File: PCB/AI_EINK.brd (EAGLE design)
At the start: 66 x 111.6 mm, 186 parts, among them IC3 WM8960, J1 BM04B-GHS-TBT(LF)(SN)(N), J2 C393939, J3 524372471, Q1 SI1308EDL-T1-GE3, Q3 NMOS_C7465427, T1 MMUN2133LT1G, U1 TPS61092RSAR, U10 AP2112-3.3K, U11 AP2112-3.3K, U12 SPU0410LR5H-QB, U2 MC74VHC1G14DFT1G, U3 BQ27441DRZR-G1A, U4 BQ24075, U5 TLV74328, U6 TLV74315, U7 TLV74318PDBVRDBV0005A_L, U8 ST25DV64K-IER6S3SOIC_IER6S3_S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, U9 EMC2301-1-ACZL-TRMSOP8_MC_MCH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, Y1 ABM8-272-T3

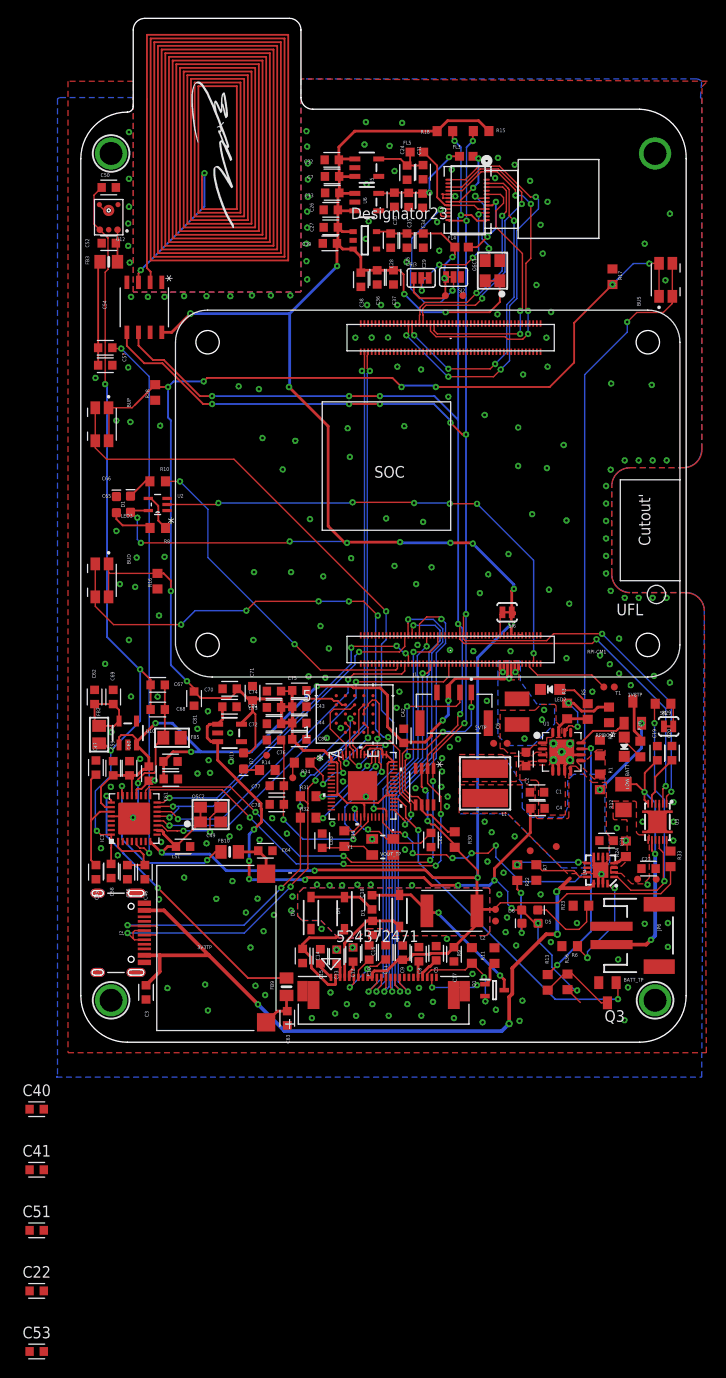
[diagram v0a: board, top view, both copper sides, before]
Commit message: PCB V3
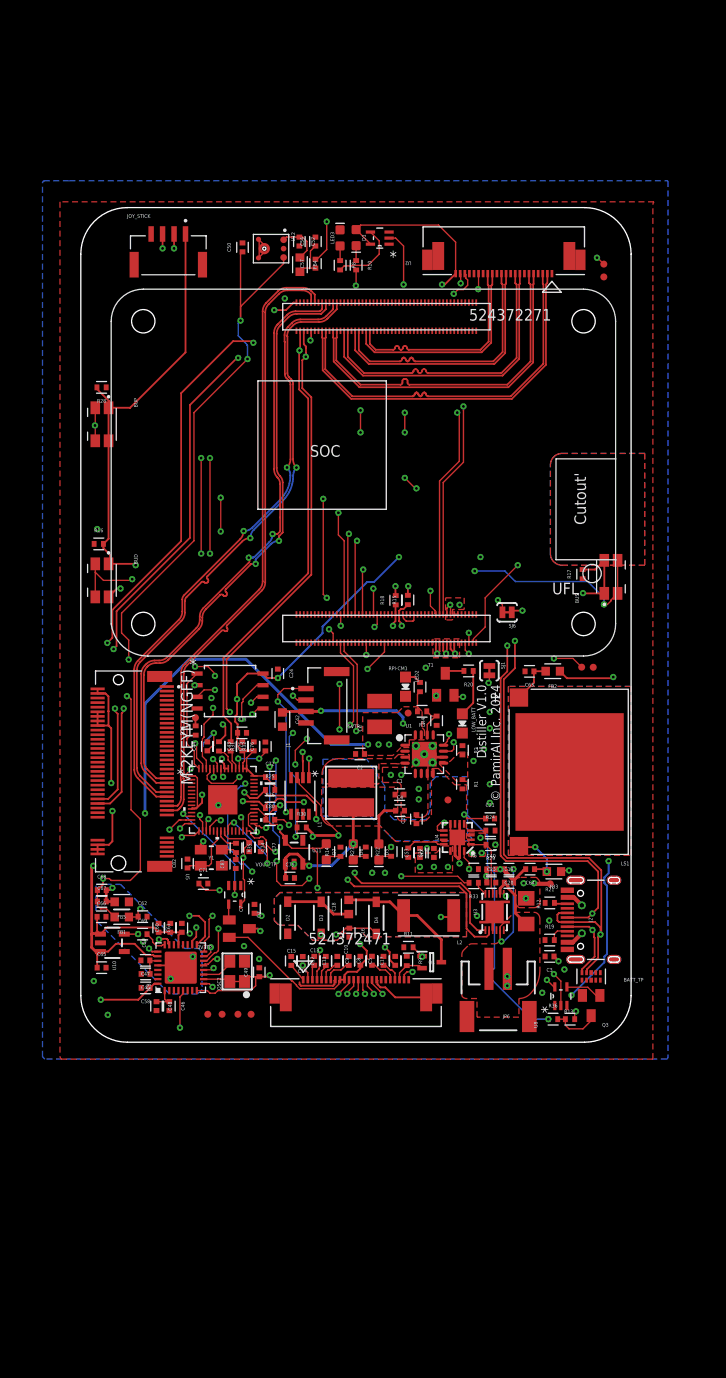
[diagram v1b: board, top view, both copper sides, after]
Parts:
- removed ANT1: NFC_ANTENNA_25X15, microbuilder:NFCANT_25X15
- removed C25, C30: 1.0uF, Capacitor:CAPC1608X85
- removed C27, C70, C78, C81: 0.1uF, Capacitor:CAPC1608X85
- removed C28, C29, C31, C32, C33, C34, C35, C36, C37, C38, C39, C41, C51: 10uF, Capacitor:CAPC1608X85
- removed FB10, FB9: 120o, microbuilder:0805-NO
- removed FL3, FL4, FL5: BLM18HE152SN1D, BLM18HE152SN1D:BEADC1608X95N
- removed GND25, RPIBOOT3: DNP, SparkFun-Connectors:PAD.03X.03
- removed J3: 524372471, 2024-02-19_09-48-43_Library:CON_524372471_MOL
- removed OSC1: 24MHz 3.3V Oscillator, microbuilder:OSC_3.2X2.5MM
- removed OV5674: DF30FC-24DS-0.4V(82)CONN_DF30FC-24DS-0.4V(82)_HIR, 2024-03-07_05-07-01_Library:CONN_DF30FC-24DS-0.4V(82)_HIR
- removed SJ2, SJ3: DNP, SparkFun-Passives:PAD-JUMPER-3-2OF3_NC_BY_TRACE_YES_SILK_FULL_BOX
- removed SPI_FLASH_SAM: W25Q128JVBIQTFBGA_128JVBIQ_WIN, 2024-03-10_02-04-46_Library:TFBGA_128JVBIQ_WIN
- removed U$10, U$11, U$94, U$95: MOUNTINGHOLE2.5, microbuilder:MOUNTINGHOLE_2.5_PLATED
- removed U7: TLV74318PDBVRDBV0005A_L, 2024-03-10_03-34-55_Library:DBV0005A_L
- added CAMERA: 524372271CON_524372271_MOL, 2024-03-29_02-21-27_Library:CON_524372271_MOL
- added EINK_524352471: 524372471, 2024-02-19_09-48-43_Library:CON_524372471_MOL
- added FB1, FB4: FERRITE_BEAD, Filter:BEADC1608X95N
- added JOY_STICK: BM04B-GHS-TBT(LF)(SN)(N), BM04B-GHS-TBT_LF__SN__N_:JST_BM04B-GHS-TBT(LF)(SN)(N)
- added M.2KEYM(NGFF): 1-2199119-5, 1-2199119-5:TE_1-2199119-5
- added Q2: NMOS_C7465427, Transistor:SOT23
- added R19: 5.1K, Resistor:RESC1005X40
- added R21: 5.1k, Resistor:RESC1005X40
- added R25, R26: 4.7K, Resistor:RESC1005X40
- added U13: TPD4EUSB30DQARDQA10, 2024-03-29_01-35-38_Library:DQA10
- C1, C10, C11, C12, C13, C14, C15, C16, C17, C19, C2, C20, C21, C22, C23, C26, C3, C4, C40, C43, C44, C45, C46, C47, C48, C49, C5, C50, C52, C53, C54, C57, C58, C59, C60, C61, C62, C63, C64, C65, C66, C67, C68, C69, C7, C71, C72, C73, C74, C75, C76, C77, C79, C8, C80, C82, C83, C9: device Capacitor:CAPC1608X85 -> Capacitor:CAPC1005X60
- C24: value 10uF -> 0.1uF; device Capacitor:CAPC1608X85 -> Capacitor:CAPC1005X60
- FB2, FB5: value Ferrite -> FERRITE_BEAD; device microbuilder:0805 -> Filter:BEADC1608X95N
- FB3: value Ferrite -> FERRITE_BEAD; device microbuilder:0805-NO -> Filter:BEADC1608X95N
- R1, R10, R11, R13, R14, R15, R16, R17, R18, R2, R20, R22, R23, R24, R28, R29, R3, R30, R31, R32, R33, R34, R35, R36, R4, R5, R6, R7, R8, R9: device resistor:R0603 -> Resistor:RESC1005X40
- U5: value TLV74328 -> MC74VHC1G14DFT1G; device adafruit_power:SOT23-5 -> MC74VHC1G14DFT1G:SOT65P210X110-5N
- U6: value TLV74315 -> W25Q128JVSIQSOIC_128JVSIQ_WIN-L; device adafruit_power:SOT23-5 -> 2024-03-29_04-43-21_Library:SOIC_128JVSIQ_WIN-L
- U8: value ST25DV64K-IER6S3SOIC_IER6S3_STM -> MC74VHC1G14DFT1G; device 2024-03-10_23-40-44_Library:SOIC_IER6S3_STM -> MC74VHC1G14DFT1G:SOT65P210X110-5N
- moved U8 87.8 mm to (53.3, 9.02), turned to 90 degrees
- moved FB3 82.3 mm to (52.6, 22.6)
- moved U5 80.6 mm to (17.8, 20.1)
- moved C7 80.3 mm to (19.9, 18.5), turned to 90 degrees
- moved RPIBOOT2 71.3 mm to (58.0, 88.8)
- moved C53 68.6 mm to (38.0, 24.6), turned to 90 degrees
- moved C26 67.1 mm to (37.6, 28.3), turned to 90 degrees
- moved GND13 65.9 mm to (58.0, 87.4)
- moved C22 64.5 mm to (39.5, 24.6), turned to 90 degrees
- moved GND 56.9 mm to (14.8, 7.05)
- moved C24 56.4 mm to (22.5, 44.2)
- moved C40 56.0 mm to (45.7, 22.9)
- moved U6 55.4 mm to (17.3, 42.3), turned to 0 degrees
- moved R15 51.7 mm to (36.7, 52.2), turned to 90 degrees
- moved R18 51.4 mm to (35.3, 52.2), turned to 90 degrees
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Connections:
- removed net 1.5V: C30.1, C34.1, C35.1, FL3.1, U6.5
- removed net 1.8V: C25.1, C28.1, C29.1, FL4.1, RPIBOOT3.P$1, SJ2.3, SJ3.1, U7.5
- removed net 2.8V: C24.1, C31.1, FL5.1, U5.5
- removed net AF_EN: OV5674.18
- removed net GPO: U8.7
- removed net N$10: FL4.2, OV5674.15
- removed net N$13: FL3.2, OV5674.13, OV5674.14
- removed net N$20: RPI-CM1.29
- removed net N$22: RPI-CM1.41
- removed net N$28: RPI-CM1.55
- removed net N$32: ANT1.P$1, U8.3
- removed net PWDN: OV5674.19, SJ3.2
- removed net RESET: OV5674.22, SJ2.2
- removed net RFC_MCLK: OSC1.3, OV5674.11
- removed net SAM_GPIO0: C2040.2
- removed net SAM_GPIO10: C2040.13
- removed net SAM_GPIO11: C2040.14
- removed net SAM_GPIO12: C2040.15
- removed net SAM_GPIO13: C2040.16
- removed net SAM_GPIO14: C2040.17
- removed net SAM_GPIO15: C2040.18
- removed net SAM_GPIO23: C2040.35
- removed net SAM_GPIO24: C2040.36
- removed net SAM_GPIO9: C2040.12
- removed net SCL: IC3.17, OV5674.23, R18.1, RPI-CM1.56, U3.2, U8.6, U9.2
- removed net SDA: IC3.18, OV5674.24, R15.1, RPI-CM1.58, U3.1, U8.5, U9.1
- removed net STROBE: OV5674.20
- removed net SYS_POW_SAM: C2040.32, Q3.1
- removed net VEH: U8.1
- new net 3V3_EINK: C17.1, C9.1, EINK_524352471.10, EINK_524352471.9, L2.1, Q2.2
- new net CAM1_C_N: CAMERA.8, RPI-CM1.127
- new net CAM1_C_P: CAMERA.9, RPI-CM1.129
- new net CAM1_D0_N: CAMERA.2, RPI-CM1.115
- new net CAM1_D0_P: CAMERA.3, RPI-CM1.117
- new net CAM1_D1_N: CAMERA.5, RPI-CM1.121
- new net CAM1_D1_P: CAMERA.6, RPI-CM1.123
- new net CAM1_D2_N: CAMERA.11, RPI-CM1.133
- new net CAM1_D2_P: CAMERA.12, RPI-CM1.135
- new net CAM1_D3_N: CAMERA.14, RPI-CM1.139
- new net CAM1_D3_P: CAMERA.15, RPI-CM1.141
- new net DSI0_C_N: RPI-CM1.169
- new net DSI0_C_P: RPI-CM1.171
- new net DSI0_D0_N: RPI-CM1.157
- new net DSI0_D0_P: RPI-CM1.159
- new net DSI0_D1_N: RPI-CM1.163
- new net DSI0_D1_P: RPI-CM1.165
- new net DSI1_C_N: RPI-CM1.187
- new net DSI1_C_P: RPI-CM1.189
- new net DSI1_D0_N: RPI-CM1.175
- new net DSI1_D0_P: RPI-CM1.177
- new net DSI1_D1_N: RPI-CM1.181
- new net DSI1_D1_P: RPI-CM1.183
- new net DSI1_D2_N: RPI-CM1.193
- new net DSI1_D2_P: RPI-CM1.195
- new net DSI1_D3_N: RPI-CM1.194
- new net DSI1_D3_P: RPI-CM1.196
- new net EXT_VCC_PCIE: M.2KEYM(NGFF).12, M.2KEYM(NGFF).14, M.2KEYM(NGFF).16, M.2KEYM(NGFF).18, M.2KEYM(NGFF).2, M.2KEYM(NGFF).4, M.2KEYM(NGFF).70, M.2KEYM(NGFF).72, M.2KEYM(NGFF).74
- new net GND_2: U13.3
- new net HDMI0_CEC: RPI-CM1.151
- new net HDMI0_CLK_N: RPI-CM1.190
- new net HDMI0_CLK_P: RPI-CM1.188
- new net HDMI0_HOTPLUG: RPI-CM1.153
- new net HDMI0_SCL: RPI-CM1.200
- new net HDMI0_SDA: RPI-CM1.199
- new net HDMI0_TX0_N: RPI-CM1.184
- new net HDMI0_TX0_P: RPI-CM1.182
- new net HDMI0_TX1_N: RPI-CM1.178
- new net HDMI0_TX1_P: RPI-CM1.176
- new net HDMI0_TX2_N: RPI-CM1.172
- new net HDMI0_TX2_P: RPI-CM1.170
- new net HDMI1_CEC: RPI-CM1.149
- new net HDMI1_CLK_N: RPI-CM1.166
- new net HDMI1_CLK_P: RPI-CM1.164
- new net HDMI1_HOTPLUG: RPI-CM1.143
- new net HDMI1_SCL: RPI-CM1.147
- new net HDMI1_SDA: RPI-CM1.145
- new net HDMI1_TX0_N: RPI-CM1.160
- new net HDMI1_TX0_P: RPI-CM1.158
- new net HDMI1_TX1_N: RPI-CM1.154
- new net HDMI1_TX1_P: RPI-CM1.152
- new net HDMI1_TX2_N: RPI-CM1.148
- new net HDMI1_TX2_P: RPI-CM1.146
- new net N$27: J2.B5, R21.2
- new net N$30: J2.A5, R19.2
- new net PCIE_!RST: M.2KEYM(NGFF).50, RPI-CM1.109
- new net PCIE_CLK_!REQ: M.2KEYM(NGFF).52, RPI-CM1.102
- new net PCIE_CLK_N: M.2KEYM(NGFF).53, RPI-CM1.112
- new net PCIE_CLK_P: M.2KEYM(NGFF).55, RPI-CM1.110
- new net PCIE_RX_N: M.2KEYM(NGFF).41, RPI-CM1.118
- new net PCIE_RX_P: M.2KEYM(NGFF).43, RPI-CM1.116
- new net PCIE_TX_N: M.2KEYM(NGFF).47, RPI-CM1.124
- new net PCIE_TX_P: M.2KEYM(NGFF).49, RPI-CM1.122
- new net RESERVED@104: RPI-CM1.104
- new net RESERVED@106: RPI-CM1.106
- new net SAM_EINK_ON: C2040.12, U5.2
- new net SAM_INTERUPT: C2040.2, RPI-CM1.46
- new net SAM_SCL: C2040.35, JOY_STICK.3, R26.1, U3.2
- new net SAM_SDA: C2040.36, JOY_STICK.2, R25.1, U3.1
- new net SCL0: CAMERA.20, RPI-CM1.80
- new net SCL1: IC3.17, R18.1, RPI-CM1.56, U9.2
- new net SDA0: CAMERA.21, RPI-CM1.82
- new net SDA1: IC3.18, R15.1, RPI-CM1.58, U9.1
- new net SYS_PI_ON: C2040.32, U8.2
- new net USB_OTG_ID: RPI-CM1.101
- new net VDAC_COMP: RPI-CM1.111
- net 3.3V: now also CAMERA.22, Q2.3; no longer C17.1, C26.1, C27.1, C32.1, C33.1, C36.1, C37.1, C38.1, C39.1, C9.1, J3.10, J3.9, L2.1, OSC1.1, OSC1.4, U5.1, U5.3, U6.1, U6.3, U7.1, U7.3, U8.8
- net AGND: now also FB5.2; no longer FB5.1
- net AVDD: now also FB1.2; no longer FB2.1
- net CAM0_C_N: no longer OV5674.8
- net CAM0_C_P: no longer OV5674.9
- net CAM0_D0_N: no longer OV5674.2
- net CAM0_D0_P: no longer OV5674.3
- net CAM0_D1_N: no longer OV5674.5
- net CAM0_D1_P: no longer OV5674.6
- net CAM_GPIO: now also CAMERA.17
- net CDD: now also EINK_524352471.7; no longer J3.7
- net EINK_BUSY: now also C2040.13, EINK_524352471.16; no longer J3.16
- net EINK_CS: now also C2040.16, EINK_524352471.13; no longer J3.13
- net EINK_D/C: now also C2040.15, EINK_524352471.14; no longer J3.14
- net EINK_RESET: now also C2040.14, EINK_524352471.15; no longer J3.15
- net GDR: now also EINK_524352471.23; no longer J3.23
- net GND: now also C24.1, CAMERA.1, CAMERA.10, CAMERA.13, CAMERA.16, CAMERA.19, CAMERA.4, CAMERA.7, EINK_524352471.17, EINK_524352471.8, EINK_524352471.P1, EINK_524352471.P2, FB5.1, JOY_STICK.4, M.2KEYM(NGFF).1, M.2KEYM(NGFF).15, M.2KEYM(NGFF).21, M.2KEYM(NGFF).27, M.2KEYM(NGFF).3, M.2KEYM(NGFF).33, M.2KEYM(NGFF).39, M.2KEYM(NGFF).45, M.2KEYM(NGFF).51, M.2KEYM(NGFF).57, M.2KEYM(NGFF).71, M.2KEYM(NGFF).73, M.2KEYM(NGFF).75, M.2KEYM(NGFF).9, M.2KEYM(NGFF).SH1, M.2KEYM(NGFF).SH2, R19.1, R21.1, U13.8, U5.3, U6.4, U8.3; no longer C24.2, C25.2, C27.2, C28.2, C29.2, C30.2, C31.2, C32.2, C33.2, C34.2, C35.2, C36.2, C37.2, C38.2, C39.2, C41.2, C51.2, C70.2, C78.2, C81.2, FB5.2, GND25.P$1, J3.17, J3.8, J3.P1, J3.P2, OSC1.2, OV5674.1, OV5674.10, OV5674.12, OV5674.21, OV5674.4, OV5674.7, SJ2.1, SJ3.3, SPI_FLASH_SAM.B3, U5.2, U6.2, U7.2, U8.4
- net LEFT_N: now also FB3.2; no longer FB10.2
- net LEFT_P: now also FB2.2; no longer FB9.2
- net N$16: now also Q3.1, U8.4; no longer ANT1.P$2, U8.2
- net N$29: now also FB4.1; no longer FB3.1
- net N$36: now also FB4.2; no longer FB3.2
- net N$40: now also FB2.1; no longer FB9.1
- net N$41: now also FB3.1; no longer FB10.1
- net N$8: now also Q2.1, U5.4; no longer FL5.2, OV5674.16, OV5674.17
- net NC: now also EINK_524352471.24; no longer J3.24
- net OUT: now also FB1.1; no longer FB2.2
- net PREVGH: now also EINK_524352471.4; no longer J3.4
- net PREVGL: now also EINK_524352471.2; no longer J3.2
- net RESE: now also EINK_524352471.22; no longer J3.22
- net SAM_1V1: no longer C78.1
- net SAM_3V3: now also C24.2, JOY_STICK.1, R25.2, R26.2, U5.5, U6.8, U8.5; no longer C70.1, C81.1, SPI_FLASH_SAM.B4
- net SAM_QSPI_SCLK: now also U6.6; no longer SPI_FLASH_SAM.B2
- net SAM_QSPI_SCN: now also U6.1; no longer SPI_FLASH_SAM.C2
- net SAM_QSPI_SD0: now also U6.5; no longer SPI_FLASH_SAM.D3
- net SAM_QSPI_SD1: now also U6.2; no longer SPI_FLASH_SAM.D2
- net SAM_QSPI_SD2: now also U6.3; no longer SPI_FLASH_SAM.C4
- net SAM_QSPI_SD3: now also U6.7; no longer SPI_FLASH_SAM.D4
- net SPI_CLK: now also C2040.17, EINK_524352471.12; no longer J3.12
- net SPI_MOSI: now also C2040.18, EINK_524352471.11; no longer J3.11
- net TSCL: now also EINK_524352471.19; no longer J3.19
- net TSDA: now also EINK_524352471.18; no longer J3.18
- net USB_N: now also U13.5
- net USB_P: now also U13.4
- net VCOM: now also EINK_524352471.1; no longer J3.1
- net VGH: now also EINK_524352471.20; no longer J3.20
- net VGL: now also EINK_524352471.21; no longer J3.21
- net VOUT: now also C26.1
- net VPP: now also EINK_524352471.6; no longer J3.6
- net VSH: now also EINK_524352471.5; no longer J3.5
- net VSL: now also EINK_524352471.3; no longer J3.3
- net V_BATT: no longer C41.1, C51.1
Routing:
- net 3.3V: track 308.1 -> 65.7 mm, vias 19 -> 15
- net SDA: track 201.4 -> 0.00 mm, vias 15 -> 0
- net SCL: track 199.3 -> 0.00 mm, vias 13 -> 0
- net RINPUT1: track 59.4 -> 185.6 mm
- net SAM_SCL: track 0.00 -> 106.1 mm, vias 0 -> 6
- net SAM_SDA: track 0.00 -> 104.0 mm, vias 0 -> 6
- net EINK_CS: track 39.7 -> 130.5 mm, vias 2 -> 3
- net EINK_BUSY: track 49.3 -> 133.9 mm, vias 2 -> 3
- net EINK_RESET: track 49.6 -> 128.3 mm, vias 2 -> 3
- net EINK_D/C: track 47.4 -> 125.7 mm, vias 2 -> 3
- net SPI_CLK: track 42.9 -> 119.8 mm, vias 2 -> 3
- net SPI_MOSI: track 44.9 -> 118.7 mm, vias 2 -> 3
- net VBUS: track 80.3 -> 9.33 mm, vias 4 -> 6
- net PCIE_!RST: track 0.00 -> 69.0 mm, vias 0 -> 4
- net PCIE_CLK_!REQ: track 0.00 -> 67.8 mm, vias 0 -> 4
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- added copper zone on layer 1, net 3.3V
- added copper zone on layer 15, net 3.3V
- added copper zone on layer 15, net 5.0V
- added copper zone on layer 16, net AGND
- added copper zone on layer 1, net BATTERY_IN
- added copper zone on layer 2, net GND
- added copper zone on layer 15, net GND1
- added copper zone on layer 2, net GND2
- added copper zone on layer 1, net GND3
- added copper zone on layer 2, net GND4
- added copper zone on layer 15, net GND5
- added copper zone on layer 16, net GND6
- added copper zone on layer 15, net SAM_3V3
- added copper zone on layer 1, net VBUS
- added copper zone on layer 15, net VBUS
- added copper zone on layer 15, net V_BATT
- removed copper zone on layer 16, net 5.0V
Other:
- board size 66 x 111.6 mm -> 60 x 91 mm
- board text added: "Distiller V1.0 © PamirAI Inc. 2024"
- board text removed: "1V8TP"
- board text removed: "RPIBOOT"
- board text removed: "Reveri H1 V1.0 © PamirAI Inc. 2024"

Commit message: pcb v4
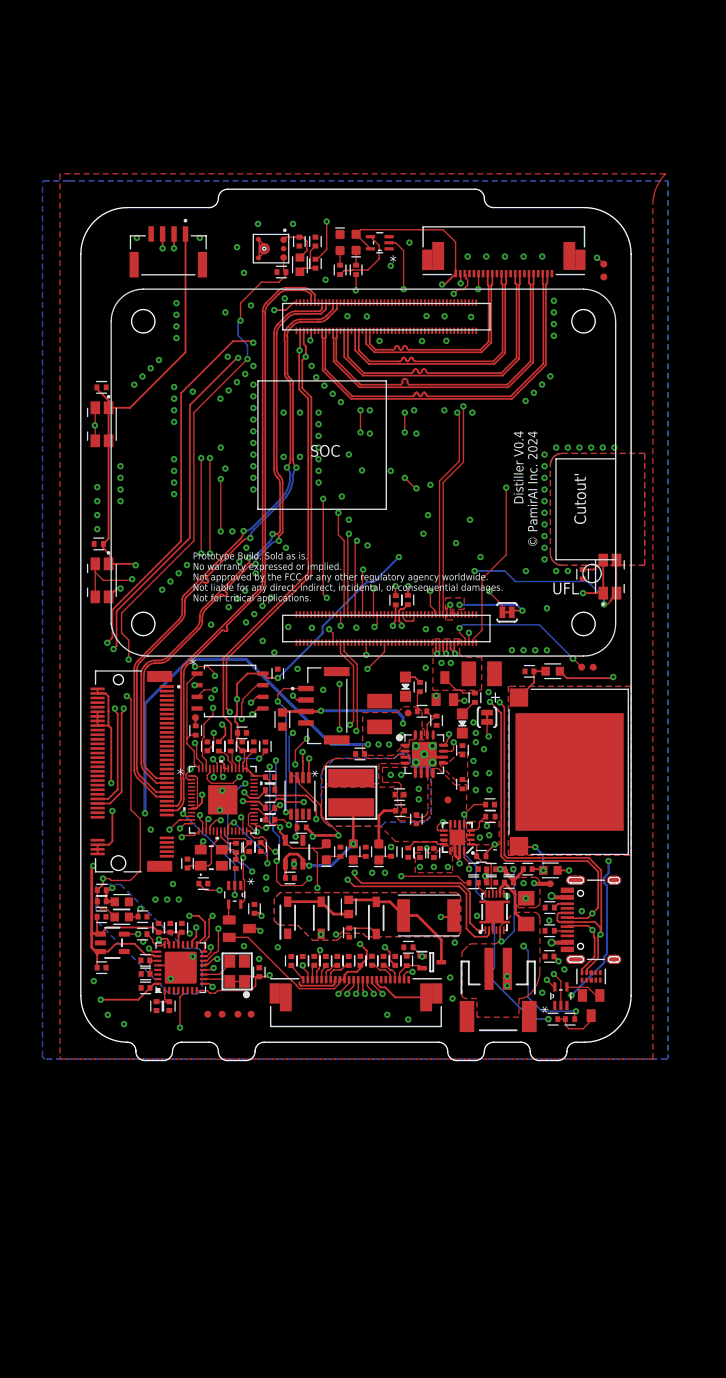
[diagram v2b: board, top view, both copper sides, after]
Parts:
- added C25: 100uF, rcl:C1210
- M.2KEYM(NGFF): value 1-2199119-5 -> 1-2199119-5 OR C841645
- U5: value MC74VHC1G14DFT1G -> MC74VHC1G14DFT1G OR C66196
- moved SJ1 5.09 mm to (45.3, 39.4)
- moved C50 5.02 mm to (22.9, 88.0), turned to 180 degrees
- moved R20 3.00 mm to (44.0, 41.6), turned to 90 degrees
- moved R29 1.63 mm to (44.7, 24.3)
- moved C21 1.52 mm to (45.6, 29.9)
- moved R24 1.52 mm to (45.7, 28.6)
- moved R19 1.02 mm to (52.1, 16.2)
- moved LED3 0.51 mm to (29.3, 91.2)
- moved R10 0.51 mm to (31.0, 88.2)
- moved R21 0.51 mm to (52.1, 18.7)
- moved D1 0.51 mm to (31.0, 91.2)
- moved R8 0.51 mm to (29.3, 88.2)
- moved U2 0.51 mm to (33.6, 91.2)
- moved T1 0.47 mm to (40.7, 42.6)
- moved FB3 0.40 mm to (52.2, 22.7)
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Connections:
- net 5.0V: now also C25.1
- net GND: now also C25.2
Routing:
- net ENABLE: track 47.3 -> 39.9 mm, vias 2 -> 3
- net 3.3V: track 65.7 -> 72.6 mm
- net AVDD: track 114.6 -> 108.3 mm
- net GND: track 48.4 -> 54.6 mm, vias 34 -> 211
- net VBUS: track 9.33 -> 5.58 mm
- net N$25: track 18.9 -> 15.5 mm
- net N$2: track 5.17 -> 1.89 mm
- net N_RPIBOOT: track 14.3 -> 17.2 mm
- net N$6: track 2.13 -> 4.41 mm
- net SAM_3V3: track 222.9 -> 220.7 mm
- net RINPUT1: track 185.6 -> 187.0 mm
- net BUTTON_U: track 67.1 -> 68.3 mm
- net !CE!: track 1.63 -> 2.67 mm
- net N$30: track 2.23 -> 1.44 mm
- net SAM_SDA: track 104.0 -> 104.7 mm
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- added copper zone on layer 2, net GND10
- added copper zone on layer 2, net GND7
- added copper zone on layer 15, net GND8
- added copper zone on layer 15, net GND9
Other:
- board size 60 x 91 mm -> 60 x 95 mm
- board text added: "Distiller V0.4 © PamirAI Inc. 2024"
- board text added: "Prototype Build. Sold as is. No warranty expressed or implied. Not approved by the FCC or any other regulatory agency worldwide. Not liable for any direct, indirect, incidental, or consequential damages. Not for critical applications."
- board text removed: "3V3TP"
- board text removed: "5VTP"
- board text removed: "BATT_TP"
- board text removed: "Distiller V1.0 © PamirAI Inc. 2024"
- board text removed: "VOUT_TP"
